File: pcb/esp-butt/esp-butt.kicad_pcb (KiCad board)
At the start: 2 copper layers, 65 x 65 mm, 18 parts, among them J1 1x04_P2.54mm, J2 JST_PH, U1 XIAO-ESP32-C3

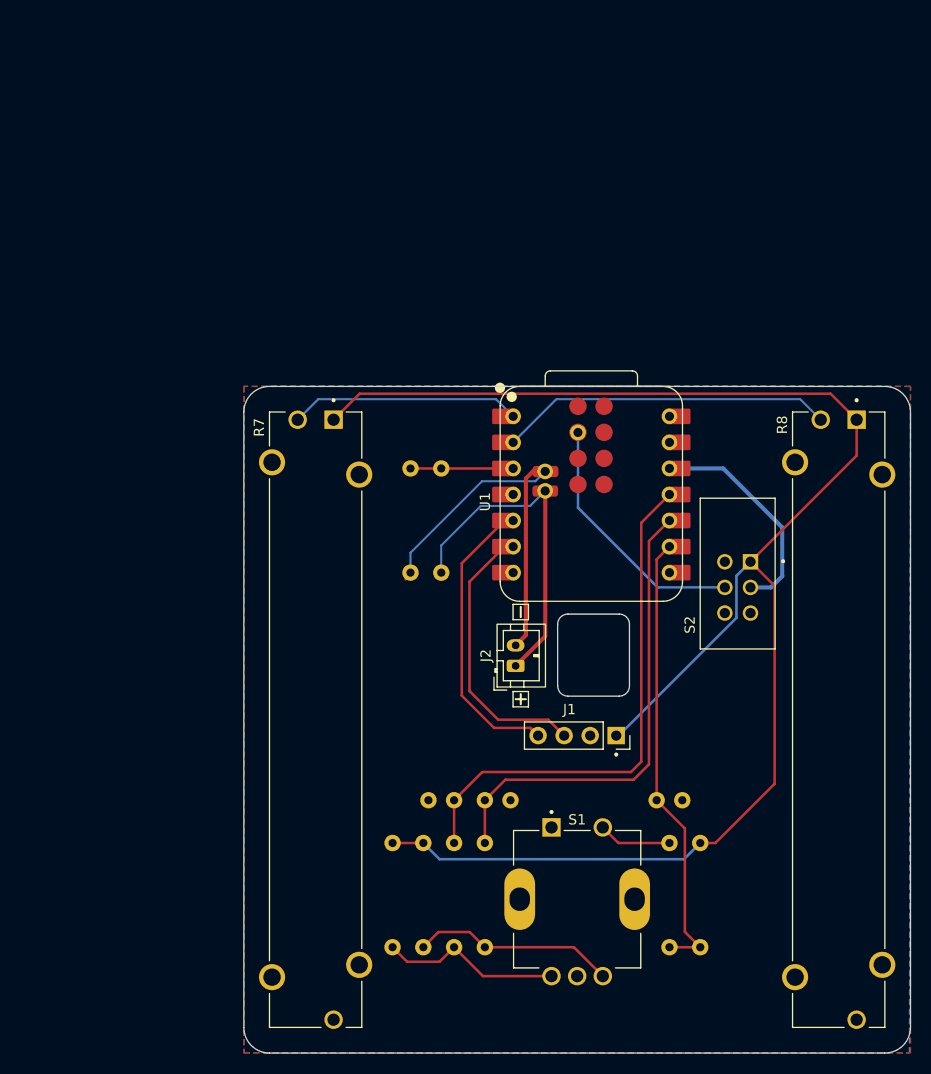
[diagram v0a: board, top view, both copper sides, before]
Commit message: More work + docs
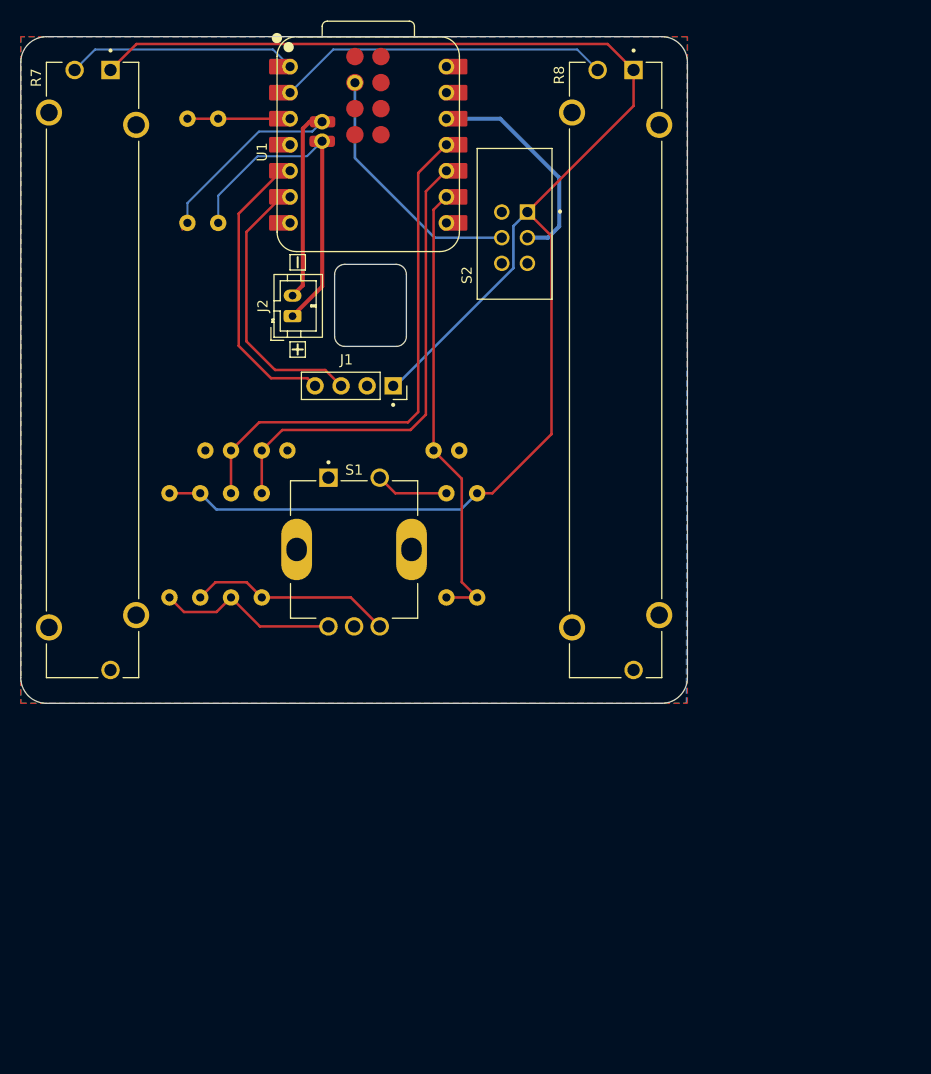
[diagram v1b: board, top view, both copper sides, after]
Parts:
- moved R1 40.4 mm to (55.8, 80.6)
- moved R5 40.4 mm to (79.8, 80.6)
- moved R6 40.4 mm to (82.8, 80.6)
- moved U1 40.4 mm to (72.1, 36.4)
- moved C1 40.4 mm to (61.8, 66.2)
- moved C2 40.4 mm to (58.8, 66.2)
- moved C3 40.4 mm to (78.5, 66.2)
- moved J1 40.4 mm to (70.8, 59.9)
- moved J2 40.4 mm to (64.8, 53.1)
- moved R10 40.4 mm to (54.5, 33.9)
- moved R2 40.4 mm to (61.8, 70.4)
- moved R3 40.4 mm to (52.8, 70.4)
- moved R4 40.4 mm to (58.8, 70.4)
- moved R7 40.4 mm to (45.2, 58.4)
- moved R8 40.4 mm to (96.2, 58.4)
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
